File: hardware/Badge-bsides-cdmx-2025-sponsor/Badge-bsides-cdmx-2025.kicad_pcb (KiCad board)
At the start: 2 copper layers, 50 x 110 mm, 30 parts, among them J1 SWDIO, J3 ADDON, J4 Conn_01x04_Pin, J5 I2C, J6 Conn_01x04_Pin, P6 USB_C_Plug_USB2.0, Q3 DMG3415U-7, SW11 ON, SW2 RESET, U1 PY32F030F28U6TR, U6 AP2112K-3.3

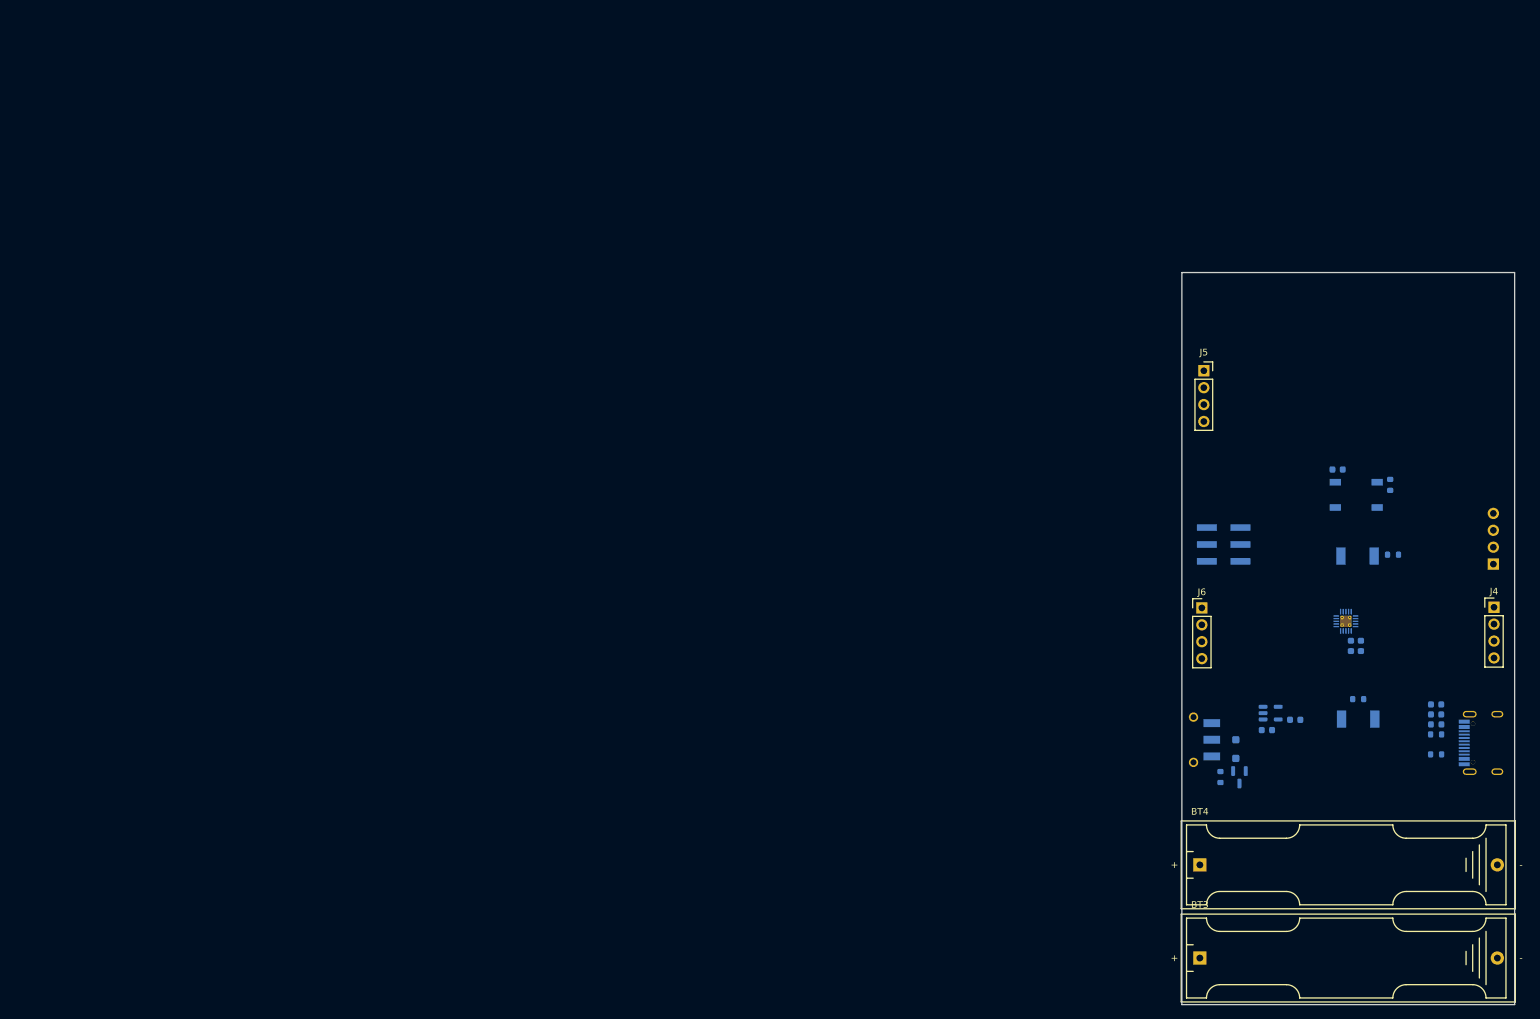
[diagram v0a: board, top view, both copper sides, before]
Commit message: feat(Hw):started_routing
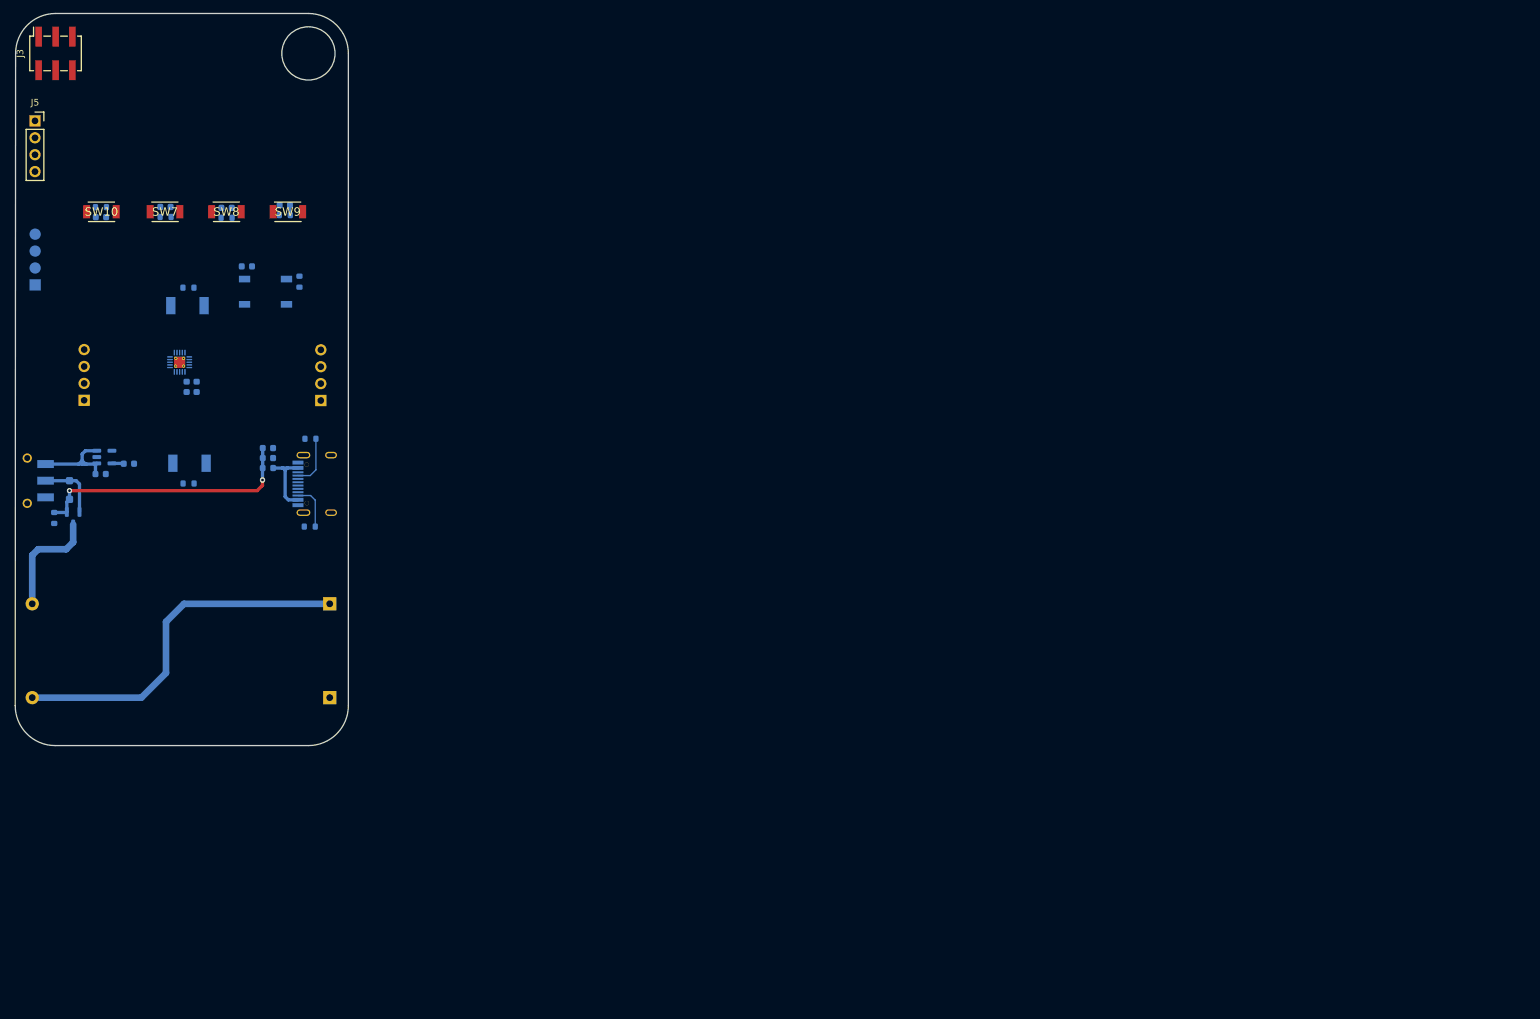
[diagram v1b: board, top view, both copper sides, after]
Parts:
- added C67: 10uF, Capacitor_SMD:C_0603_1608Metric, B.Cu at (-18.5, 29.3)
- added C68: 10uF, Capacitor_SMD:C_0603_1608Metric, B.Cu at (-9.79, 28.9)
- added C69: 10uF, Capacitor_SMD:C_0603_1608Metric, B.Cu at (-27.7, 29.1)
- added C70: 10uF, Capacitor_SMD:C_0603_1608Metric, B.Cu at (-37.4, 30.7)
- added R5: 10k, Resistor_SMD:R_0603_1608Metric, B.Cu at (-18.5, 30.8)
- added R6: 10k, Resistor_SMD:R_0603_1608Metric, B.Cu at (-9.79, 30.4)
- added R7: 10k, Resistor_SMD:R_0603_1608Metric, B.Cu at (-27.7, 30.6)
- added R8: 10k, Resistor_SMD:R_0603_1608Metric, B.Cu at (-37.4, 29.2)
- added SW10: SW_Push, Footprints:TS1088R02026, F.Cu at (-37.3, 29.9)
- added SW7: SW_Push, Footprints:TS1088R02026, F.Cu at (-27.8, 29.9)
- added SW8: SW_Push, Footprints:TS1088R02026, F.Cu at (-18.6, 29.9)
- added SW9: SW_Push, Footprints:TS1088R02026, F.Cu at (-9.34, 29.9)
- BT3, BT4: moved to B.Cu
- J3: moved to F.Cu
- J4: footprint Connector_PinHeader_2.54mm:PinHeader_1x04_P2.54mm_Vertical -> Connector_PinHeader_2.54mm:PinHeader_1x04_P2.54mm_Horizontal; moved to B.Cu
- J6: footprint Connector_PinHeader_2.54mm:PinHeader_1x04_P2.54mm_Vertical -> Connector_PinSocket_2.54mm:PinSocket_1x04_P2.54mm_Horizontal; moved to B.Cu
- moved J1 223.1 mm to (-47.3, 40.9)
- moved J3 190.4 mm to (-44.2, 6.08), turned to 90 degrees
- moved R11 185.4 mm to (-24.3, 41.3), turned to 180 degrees
- moved C33 180.0 mm to (-12.3, 65.4)
- moved D10 179.8 mm to (-24.4, 44.0)
- moved D9 179.8 mm to (-24.1, 67.7), turned to 0 degrees
- moved F3 179.7 mm to (-12.3, 68.4)
- moved J5 179.6 mm to (-47.3, 16.2)
- moved D4 179.5 mm to (-42.1, 71.7)
- moved P6 179.5 mm to (-6.99, 70.8)
- moved Q3 179.5 mm to (-41.6, 75.9)
- moved R10 179.5 mm to (-44.4, 75.9)
- moved SW11 179.5 mm to (-46.7, 70.3)
- moved U1 179.5 mm to (-25.6, 52.5)
- moved C10 179.4 mm to (-37.5, 69.3)
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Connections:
- BT3 pad 2: +3.3V -> +BATT
- J3 pad 5: /GPIO1 -> /GPIO2
- J3 pad 6: /GPIO2 -> /GPIO1
- J4 pad 1: /RX -> GND
- J4 pad 2: /RX -> GND
- J4 pad 3: GND -> /RX
- J4 pad 4: GND -> /RX
- J6 pad 1: /TX -> GND
- J6 pad 2: /TX -> GND
- J6 pad 3: GND -> /TX
- J6 pad 4: GND -> /TX
- U1 pad 1: unconnected-(U1-PA5-Pad1) -> /BTTN2
- U1 pad 10: unconnected-(U1-PB6-Pad10) -> /LED1
- U1 pad 16: /GPIO2 -> /BTTN4
- U1 pad 17: /GPIO1 -> /BTTN3
- U1 pad 2: /LED1 -> /BTTN1
- U1 pad 20: unconnected-(U1-PA4-Pad20) -> /LED2
- U1 pad 3: /LED2 -> /GPIO1
- U1 pad 5: unconnected-(U1-PA12-Pad5) -> /GPIO2
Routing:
- net Net-(BT3--): track 0.00 -> 55.1 mm
- net VBUS: track 0.00 -> 40.2 mm, vias 0 -> 2
- net +BATT: track 0.00 -> 16.9 mm
- net Net-(SW11-A): track 0.00 -> 14.8 mm
- net Net-(F3-Pad1): track 0.00 -> 10.8 mm
- net Net-(D4-K): track 0.00 -> 9.51 mm
- net Net-(P6-CC): track 0.00 -> 7.73 mm
- net Net-(P6-VCONN): track 0.00 -> 6.86 mm
- net +3V3: track 0.00 -> 1.80 mm
- net /BTTN2: track 0.00 -> 1.52 mm
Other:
- board size 50 x 110 mm -> 50.1 x 110 mm
